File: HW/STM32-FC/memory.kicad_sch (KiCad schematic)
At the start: 2 parts, among them U5 W25X40CLSN

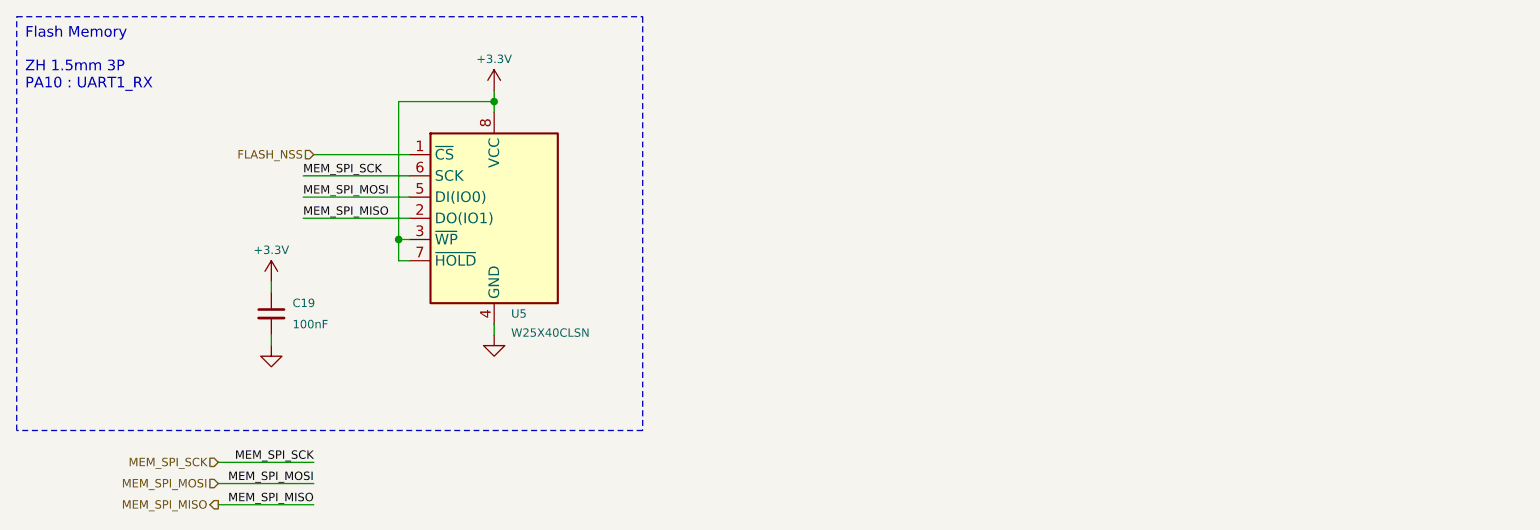
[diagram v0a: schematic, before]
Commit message: Baro/SD Card update
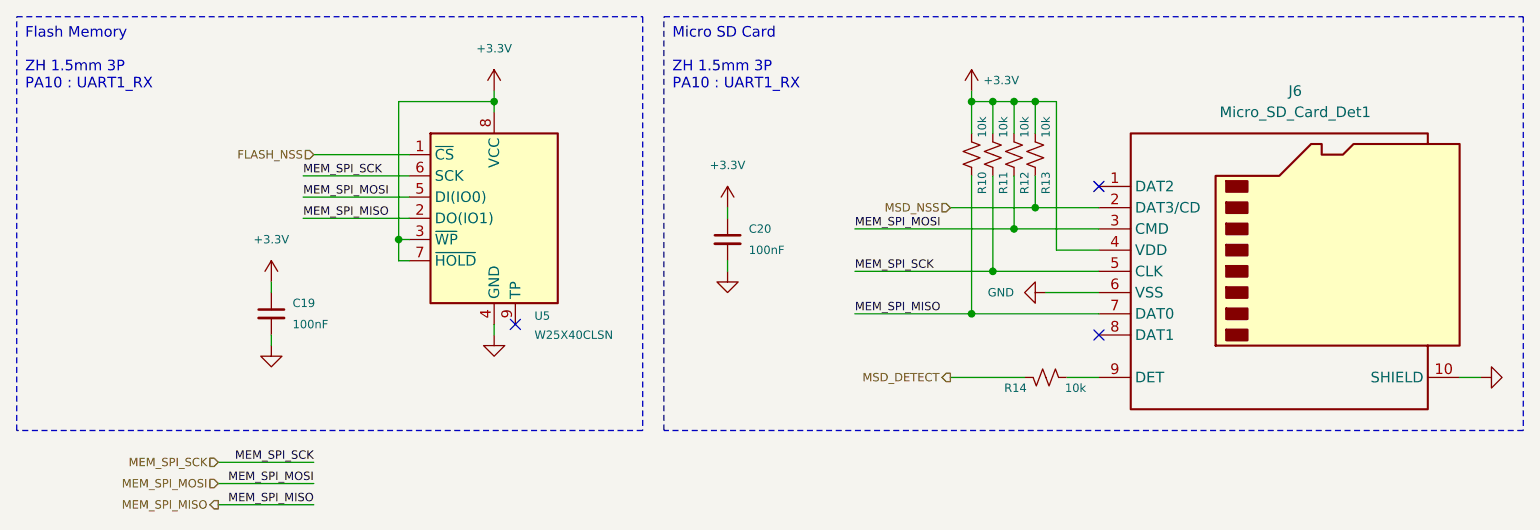
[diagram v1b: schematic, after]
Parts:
- added C20: 100nF, Capacitor_SMD:C_0402_1005Metric, symbol Device:C_Small
- added J6: Micro_SD_Card_Det1, Connector_Card:microSD_HC_Molex_104031-0811, symbol Connector:Micro_SD_Card_Det1
- added R10, R11, R12, R13, R14: 10k, Resistor_SMD:R_0402_1005Metric, symbol Device:R_Small_US
- U5: footprint Package_SO:SOIC-8_3.9x4.9mm_P1.27mm -> W25X40CLUX:USON_LUXIG_TR_HandSolder; symbol Memory_Flash:W25X40CLSN -> W25X40CLUX:W25X40CLUX
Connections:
- net +3.3V: now also C20.1, J6.4 (VDD), R10.1, R11.1, R12.1, R13.1
- net GND: now also C20.2, J6.10 (SHIELD), J6.6 (VSS)
- net MEM_SPI_MISO: now also J6.7 (DAT0), R10.2
- net MEM_SPI_MOSI: now also J6.3 (CMD), R12.2
- net MEM_SPI_SCK: now also J6.5 (CLK), R11.2
- new net: J6.9 (DET), R14.2
- new net MSD_DETECT: R14.1
- new net MSD_NSS: J6.2 (DAT3/CD), R13.2
- no-connect marks 0 -> 3
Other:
- note added: "Micro SD Card"
